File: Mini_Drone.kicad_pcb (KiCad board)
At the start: 4 copper layers, 30 parts, among them J1 Conn_01x02, Q1 AO3400A, Q2 AO3400A, Q3 AO3400A, Q4 AO3400A, U1 XIAO ESP32-S3, U2 MPU-6050

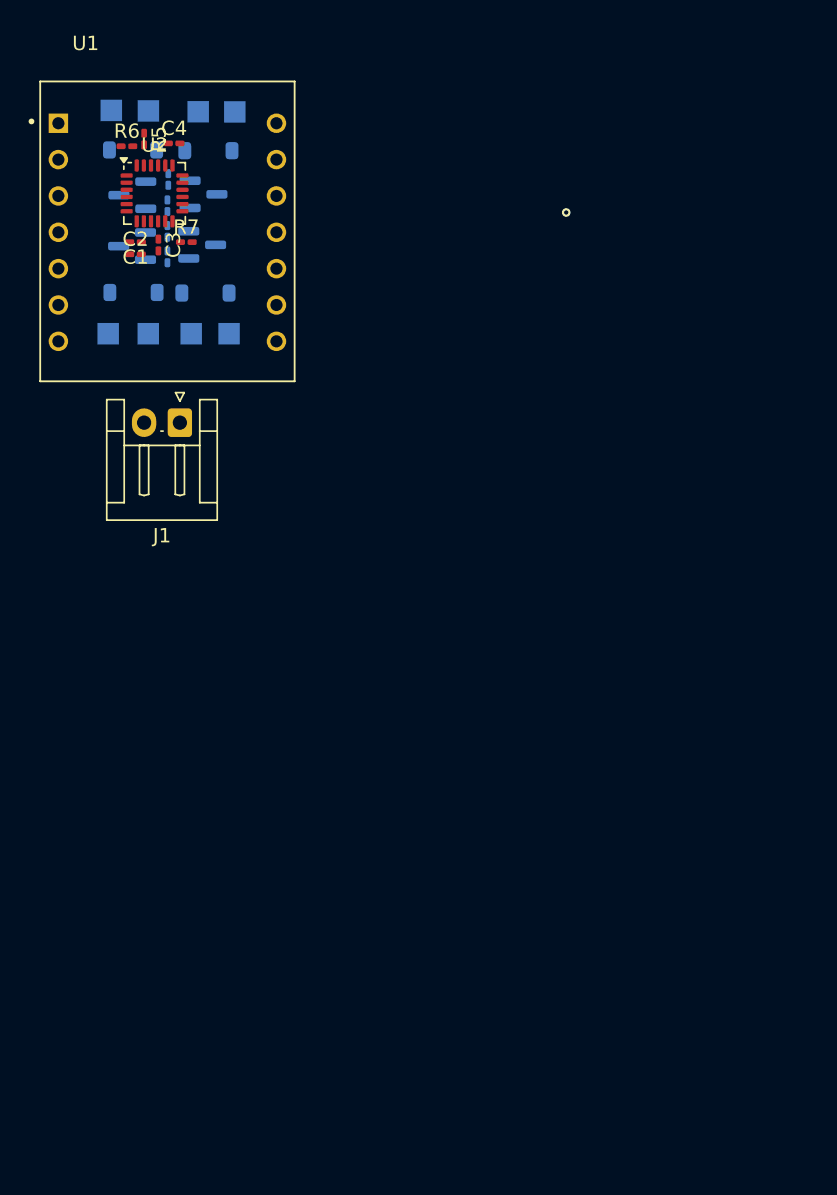
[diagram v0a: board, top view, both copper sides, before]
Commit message: 1 unconnected
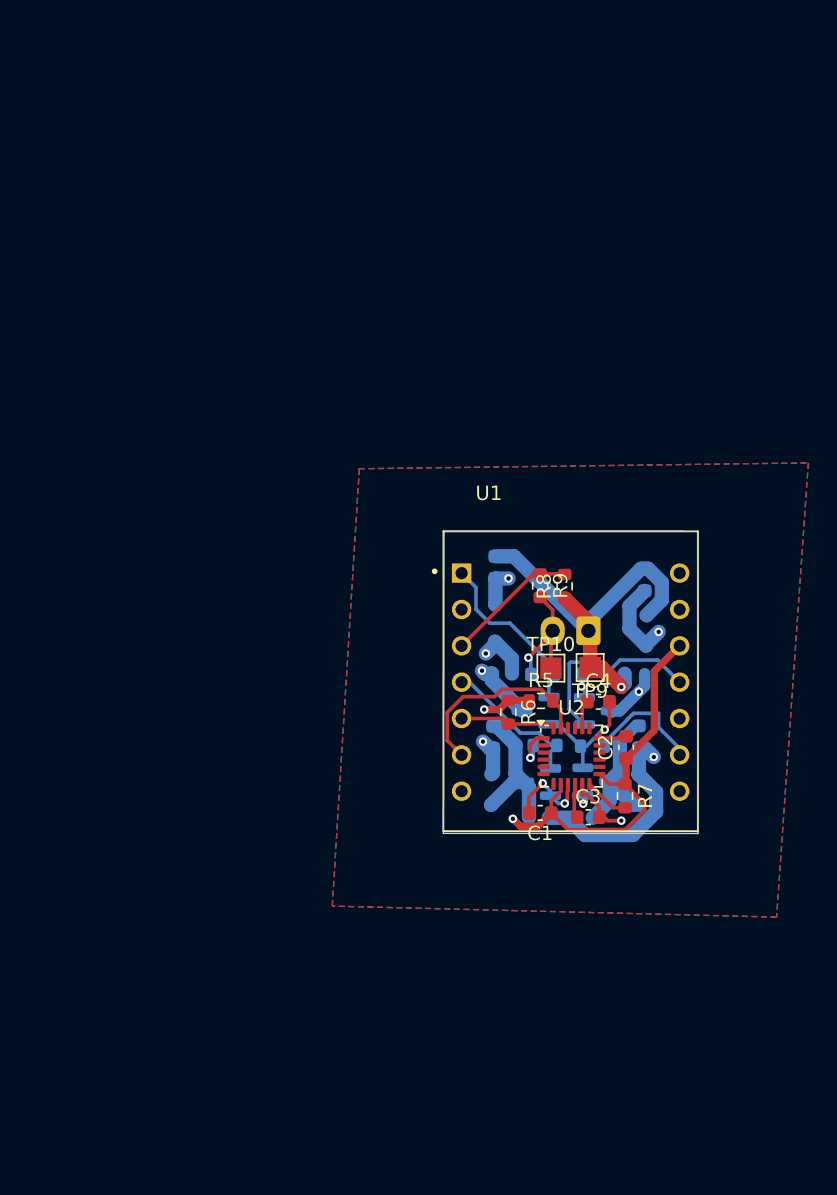
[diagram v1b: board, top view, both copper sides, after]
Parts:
- removed D4: 1N4148W, Diode_SMD:D_SOD-123
- added C5: 1uf, Capacitor_SMD:C_0603_1608Metric, B.Cu at (124.8, 121.2)
- added C6: 1uf, Capacitor_SMD:C_0603_1608Metric, B.Cu at (135.2, 122.0)
- added C7: 1uf, Capacitor_SMD:C_0603_1608Metric, B.Cu at (124.6, 133.0)
- added C8: 1uf, Capacitor_SMD:C_0603_1608Metric, B.Cu at (134.8, 133.0)
- added D2: 1N4148WT, Diode_SMD:D_SOD-523, B.Cu at (127.8, 138.6)
- added R8: 10k, Resistor_SMD:R_0603_1608Metric, F.Cu at (129.6, 122.5)
- added R9: 10k, Resistor_SMD:R_0603_1608Metric, F.Cu at (127.9, 122.5)
- added TP10: TestPoint, TestPoint:TestPoint_Pad_1.5x1.5mm, F.Cu at (128.6, 128.2)
- added TP9: TestPoint, TestPoint:TestPoint_Pad_1.5x1.5mm, F.Cu at (131.4, 128.2)
- C1, C2, C3, C4: footprint Capacitor_SMD:C_0201_0603Metric_Pad0.64x0.40mm_HandSolder -> Capacitor_SMD:C_0603_1608Metric
- D1, D3, D5: value 1N4148W -> 1N4148WT; footprint Diode_SMD:D_SOD-123 -> Diode_SMD:D_SOD-523
- J1: moved to B.Cu
- R1, R2, R3, R4, R5, R6, R7: value R -> 10k; footprint Resistor_SMD:R_0201_0603Metric_Pad0.64x0.40mm_HandSolder -> Resistor_SMD:R_0603_1608Metric
- TP1, TP2, TP3, TP4, TP5, TP6, TP7, TP8: footprint TestPoint:TestPoint_Pad_1.5x1.5mm -> TestPoint:TestPoint_Pad_D1.0mm
- moved TP8 57.4 mm to (134.8, 137.8)
- moved TP7 55.3 mm to (124.5, 137.8), turned to -90 degrees
- moved TP4 54.2 mm to (134.8, 135.6)
- moved D3 53.5 mm to (130.8, 138.7)
- moved TP3 52.2 mm to (124.5, 135.6), turned to -90 degrees
- moved D1 50.7 mm to (134.5, 128.6), turned to 0 degrees
- moved C3 50.0 mm to (131.2, 138.6), turned to 0 degrees
- moved Q3 49.8 mm to (127.7, 136.2)
- moved R7 49.4 mm to (133.8, 137.1), turned to -90 degrees
- moved Q4 49.4 mm to (131.8, 136.1)
- moved C4 49.0 mm to (131.9, 130.6)
- moved U2 48.9 mm to (130.1, 134.4)
- moved C1 48.9 mm to (127.9, 138.3)
- moved C2 48.6 mm to (133.9, 133.8), turned to 90 degrees
- moved R5 48.1 mm to (127.9, 130.5), turned to 0 degrees
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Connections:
- Q1 pad 3: Net-(D4-A) -> Net-(D5-A)
- Q2 pad 1: /D1 -> /D10
- Q2 pad 3: Net-(D5-A) -> Net-(D1-A)
- Q3 pad 1: /D2 -> /D3
- Q3 pad 3: Net-(D1-A) -> Net-(D2-A)
- Q4 pad 1: /D3 -> /D8
- R2 pad 1: /D1 -> /D10
- R3 pad 1: /D2 -> /D3
- R4 pad 1: /D3 -> /D8
- TP5 pad 1: Net-(D4-A) -> Net-(D5-A)
- TP6 pad 1: Net-(D5-A) -> Net-(D1-A)
- TP7 pad 1: Net-(D1-A) -> Net-(D2-A)
- U1 pad 11: unconnected-(U1-D10-Pad11) -> /D10
- U1 pad 9: unconnected-(U1-D8-Pad9) -> /D8
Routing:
- net /BAT+: track 0.00 -> 50.2 mm, vias 0 -> 4
- net +3V3: track 0.00 -> 40.8 mm, vias 0 -> 2
- net GND: track 0.00 -> 36.6 mm, vias 0 -> 7
- net /D8: track 0.00 -> 18.0 mm, vias 0 -> 1
- net Net-(D5-A): track 0.00 -> 15.3 mm, vias 0 -> 2
- net Net-(D1-A): track 0.00 -> 14.7 mm, vias 0 -> 2
- net /SCL: track 0.00 -> 13.9 mm
- net /D10: track 0.00 -> 13.8 mm
- net /D0: track 0.00 -> 12.3 mm
- net Net-(D3-A): track 0.00 -> 10.6 mm
- net Net-(D2-A): track 0.00 -> 10.5 mm
- net /D3: track 0.00 -> 10.3 mm
- net /D2: track 0.00 -> 9.30 mm
- net /SDA: track 0.00 -> 6.71 mm
- net Net-(U2-INT): track 0.00 -> 3.18 mm
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- added copper zone on In2.Cu, net /BAT+
- added copper zone on B.Cu, net GND
- added copper zone on F.Cu, net GND
- added copper zone on In1.Cu, net GND
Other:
- board outline added: 17.8 x 21.1 mm

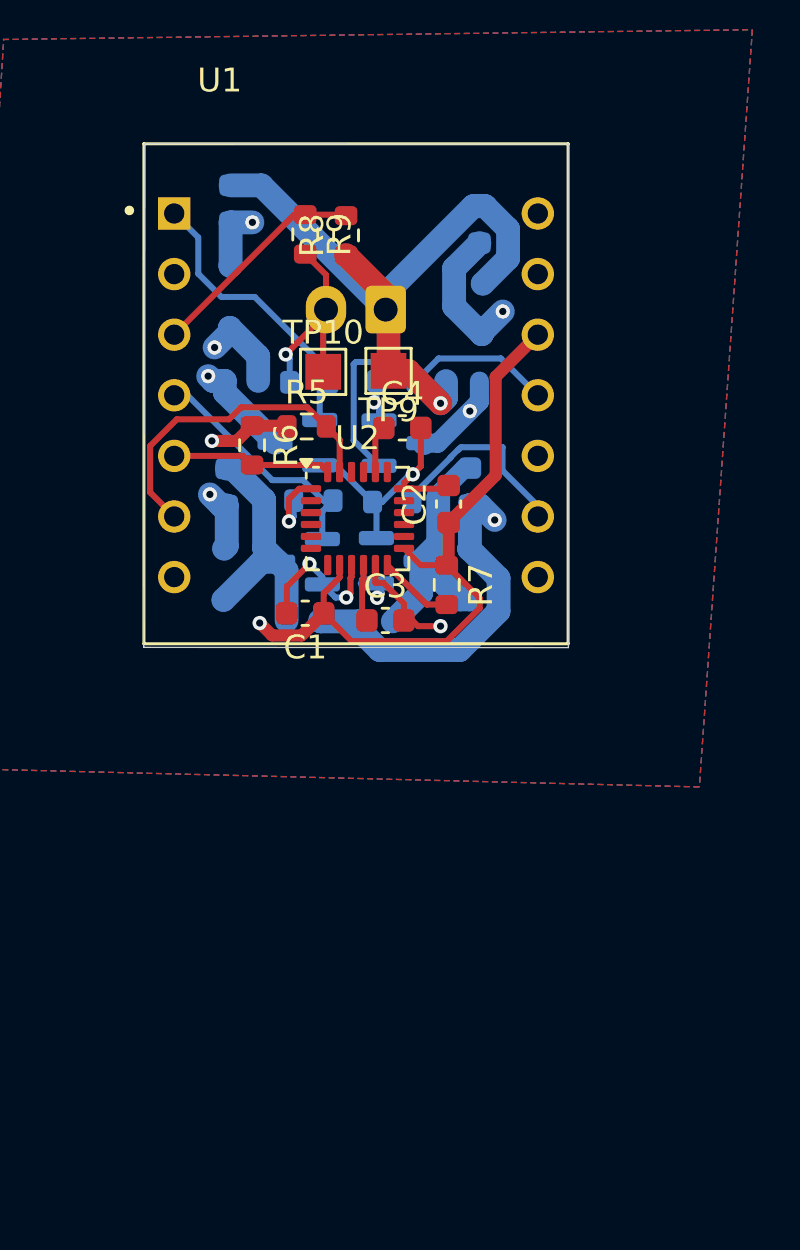
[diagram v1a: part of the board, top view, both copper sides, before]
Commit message: good progress
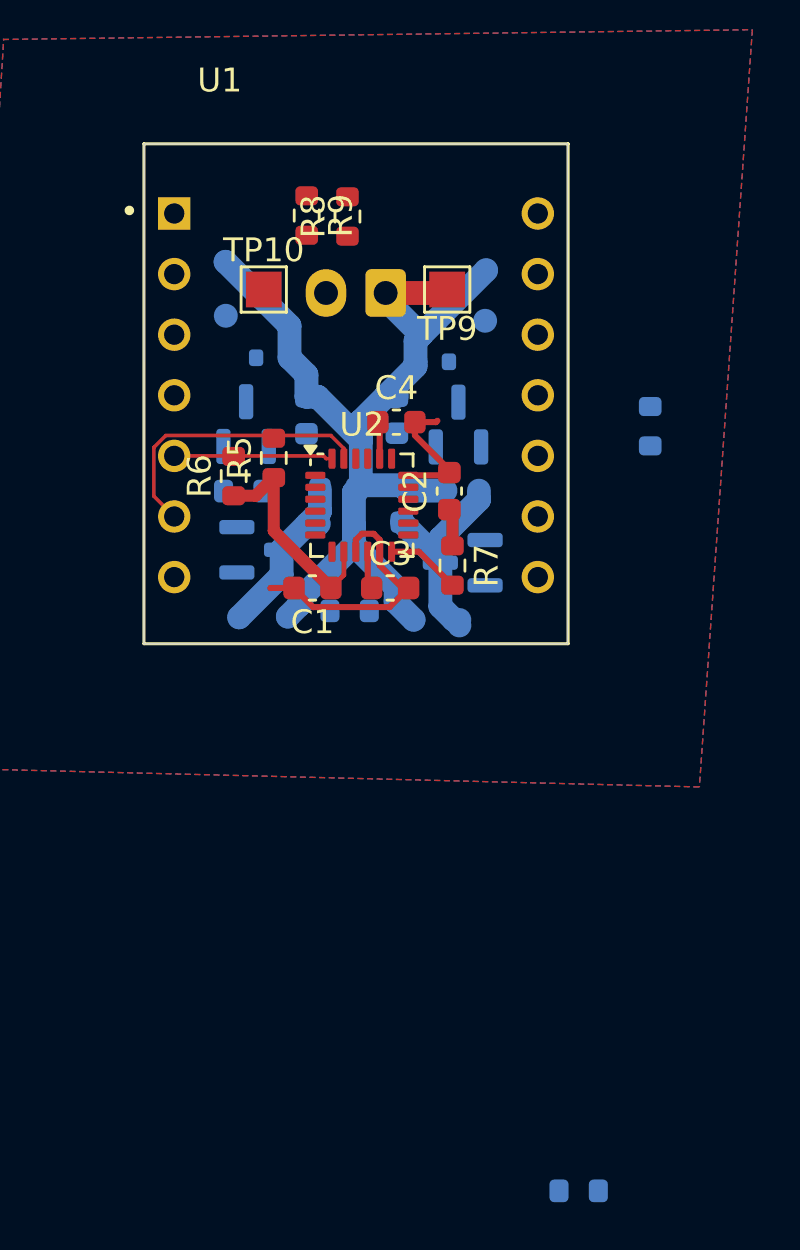
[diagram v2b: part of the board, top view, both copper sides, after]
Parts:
- U2: footprint Sensor_Motion:InvenSense_QFN-24_4x4mm_P0.5mm -> Drone_prj:InvenSense_QFN-24_4x4mm_P0.5mm
- moved R4 29.9 mm to (139.3, 162.5)
- moved R2 10.8 mm to (142.3, 130.5), turned to 90 degrees
- moved C5 9.41 mm to (127.9, 130.0)
- moved C6 8.69 mm to (131.7, 130.0)
- moved D3 6.56 mm to (134.5, 133.2)
- moved R1 5.34 mm to (125.3, 133.2), turned to 0 degrees
- moved R3 4.86 mm to (129.7, 138.2), turned to 0 degrees
- moved C7 4.68 mm to (129.3, 133.1), turned to 180 degrees
- moved TP10 4.25 mm to (126.1, 124.8)
- moved D2 4.24 mm to (129.2, 134.7)
- moved TP9 4.20 mm to (133.8, 124.8)
- moved TP3 3.91 mm to (127.2, 138.5), turned to 0 degrees
- moved TP4 3.77 mm to (132.4, 138.6), turned to 90 degrees
- moved C8 2.94 mm to (131.9, 133.7), turned to -90 degrees
- moved TP1 2.78 mm to (124.5, 123.6)
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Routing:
- net +3V3: track 40.8 -> 10.9 mm, vias 2 -> 0
- net GND: track 36.6 -> 16.3 mm, vias 7 -> 0
- net /D8: track 18.0 -> 0.00 mm, vias 1 -> 0
- net Net-(D5-A): track 15.3 -> 0.00 mm, vias 2 -> 0
- net Net-(D1-A): track 14.7 -> 0.00 mm, vias 2 -> 0
- net /D10: track 13.8 -> 0.00 mm
- net /D0: track 12.3 -> 0.00 mm
- net /D3: track 10.3 -> 0.00 mm
- net /D2: track 9.30 -> 0.00 mm
- net /BAT+: track 50.2 -> 41.4 mm, vias 4 -> 0
- net Net-(D2-A): track 10.5 -> 7.24 mm
- net /SCL: track 13.9 -> 12.1 mm
- net Net-(D3-A): track 10.6 -> 8.92 mm
- net Net-(U2-REGOUT): track 2.71 -> 1.59 mm
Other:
- board size 17.8 x 21.1 mm -> 17.8 x 21 mm

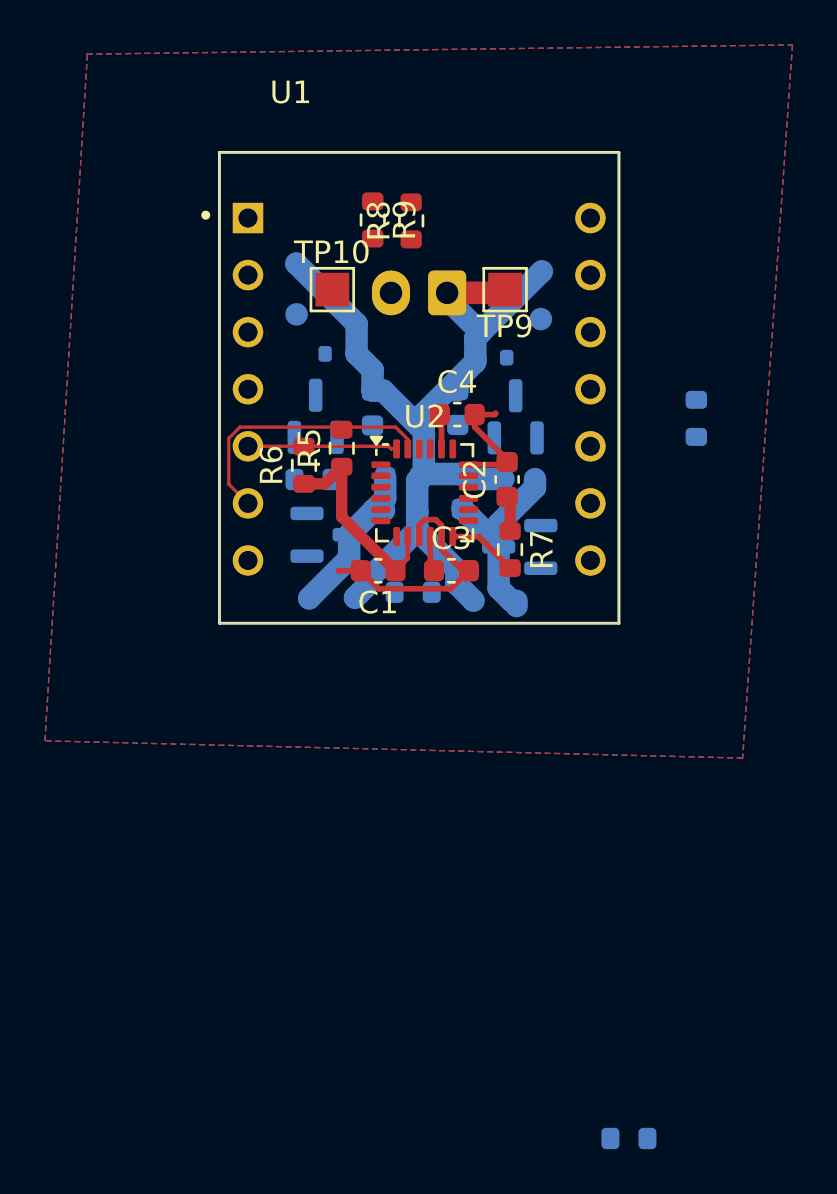
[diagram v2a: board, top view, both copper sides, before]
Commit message: no errors success
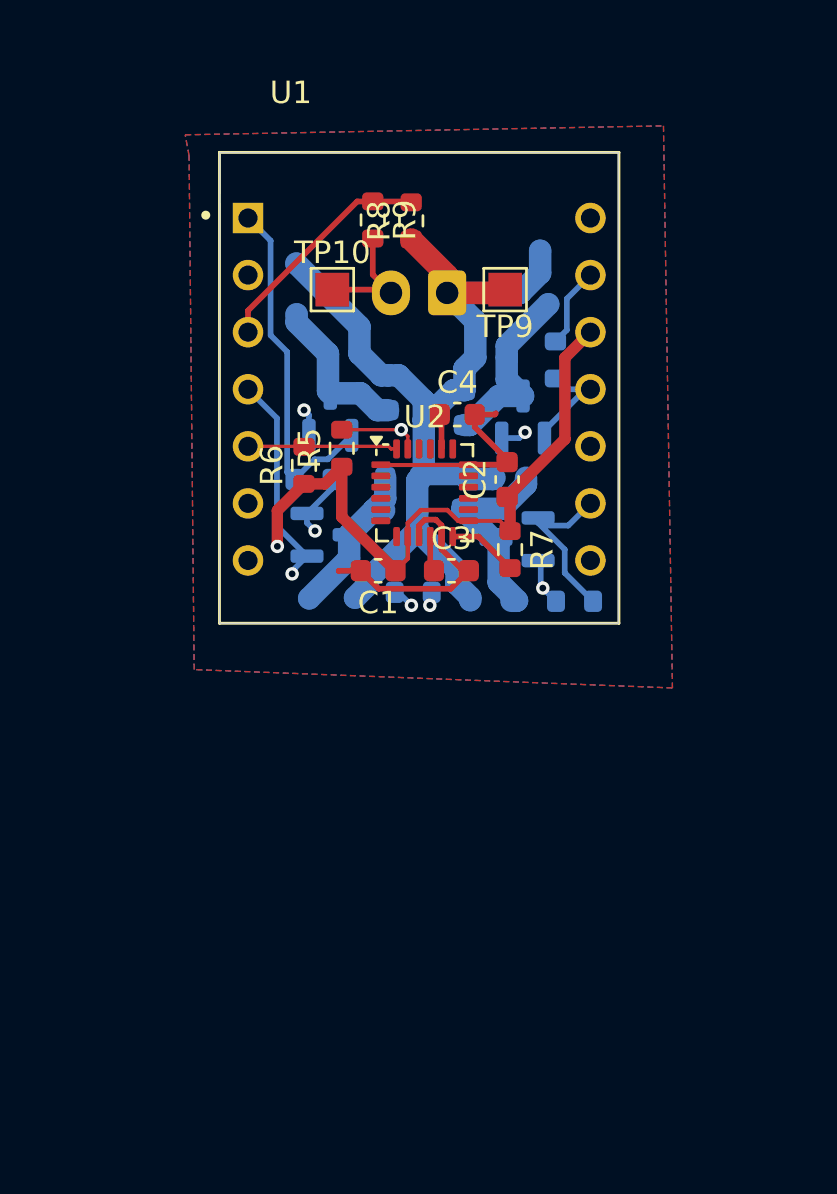
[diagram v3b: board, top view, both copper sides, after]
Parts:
- moved R4 24.0 mm to (136.9, 138.6)
- moved R2 6.79 mm to (136.1, 127.9)
- moved C5 0.97 mm to (128.6, 129.3)
- moved TP2 0.93 mm to (135.4, 123.0)
- moved TP6 0.74 mm to (135.8, 125.4)
- moved Q1 0.66 mm to (126.0, 130.3)
- moved D3 0.40 mm to (134.1, 133.1)
- moved Q4 0.36 mm to (134.4, 135.9)
- moved Q2 0.33 mm to (134.6, 130.4)
- moved C6 0.30 mm to (132.0, 130.0)
- moved TP8 0.24 mm to (134.4, 138.6)
- moved TP4 0.14 mm to (132.3, 138.6)
- moved D5 0.13 mm to (126.6, 127.6)
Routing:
- net +3V3: track 10.9 -> 46.8 mm, vias 0 -> 1
- net GND: track 16.3 -> 39.3 mm, vias 0 -> 5
- net /D3: track 0.00 -> 16.5 mm, vias 0 -> 2
- net /D0: track 0.00 -> 15.9 mm
- net /D2: track 0.00 -> 10.3 mm
- net Net-(D1-A): track 0.00 -> 8.29 mm
- net /D8: track 0.00 -> 7.60 mm
- net Net-(D5-A): track 0.00 -> 7.02 mm
- net /D10: track 0.00 -> 4.56 mm
- net /BAT+: track 41.4 -> 44.9 mm
- net /SCL: track 12.1 -> 11.8 mm, vias 0 -> 1
